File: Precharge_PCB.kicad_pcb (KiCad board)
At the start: 4 copper layers, 146 parts, among them J1 Conn_01x02, J2 Conn_01x02, J3 Conn_01x02, J4 Conn_01x02, J5 Conn_01x08, J6 Conn_01x03, J7 Conn_01x04, J8 Conn_01x04, J9 Conn_01x06, K1 G2RL-1A, K2 G2RL-1A, K3 G9KB-1A, K4 SPU01M-05, Q1 DMN61D8LQ, Q2 DMN61D8LQ, Q3 DMN61D8LQ, Q4 DMN61D8LQ, Q5 DMN61D8LQ, Q6 DMN61D8LQ, Q7 DMN61D8LQ, Q8 DMN61D8LQ, SW1 SW_Push, U1 TPS7B88, U2 MCP1700x-330xxMB, U3 STM32F103C8Tx, U4 SN65HVD1050D, U5 LM393, U6 4N35, U7 AMC1351, U8 AMC1351, U9 TLV6002, Y1 8M

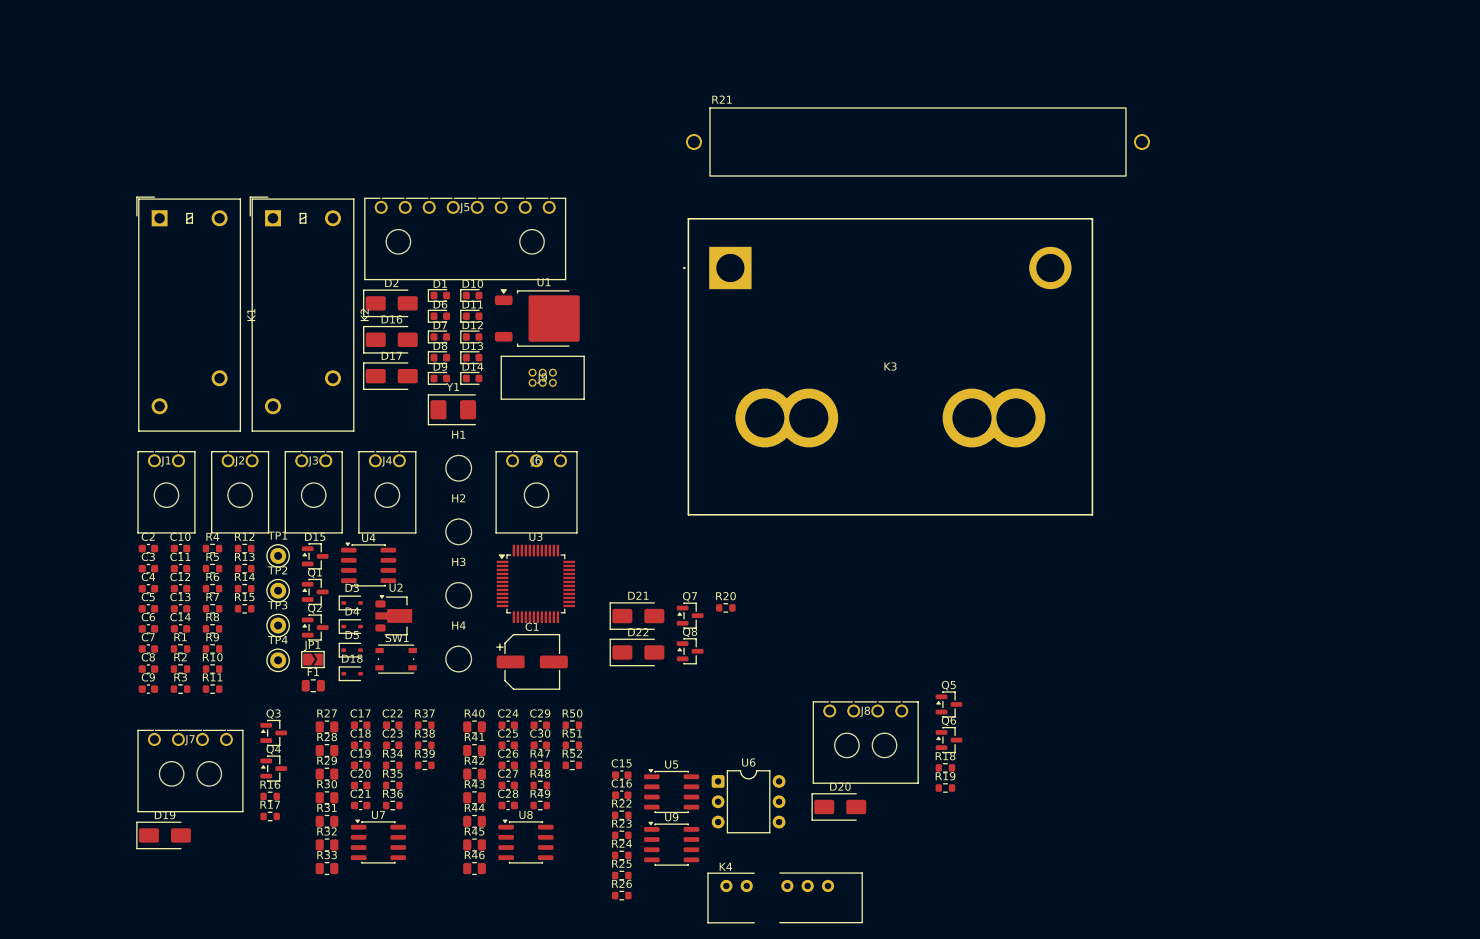
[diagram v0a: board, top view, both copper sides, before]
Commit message: Revision A
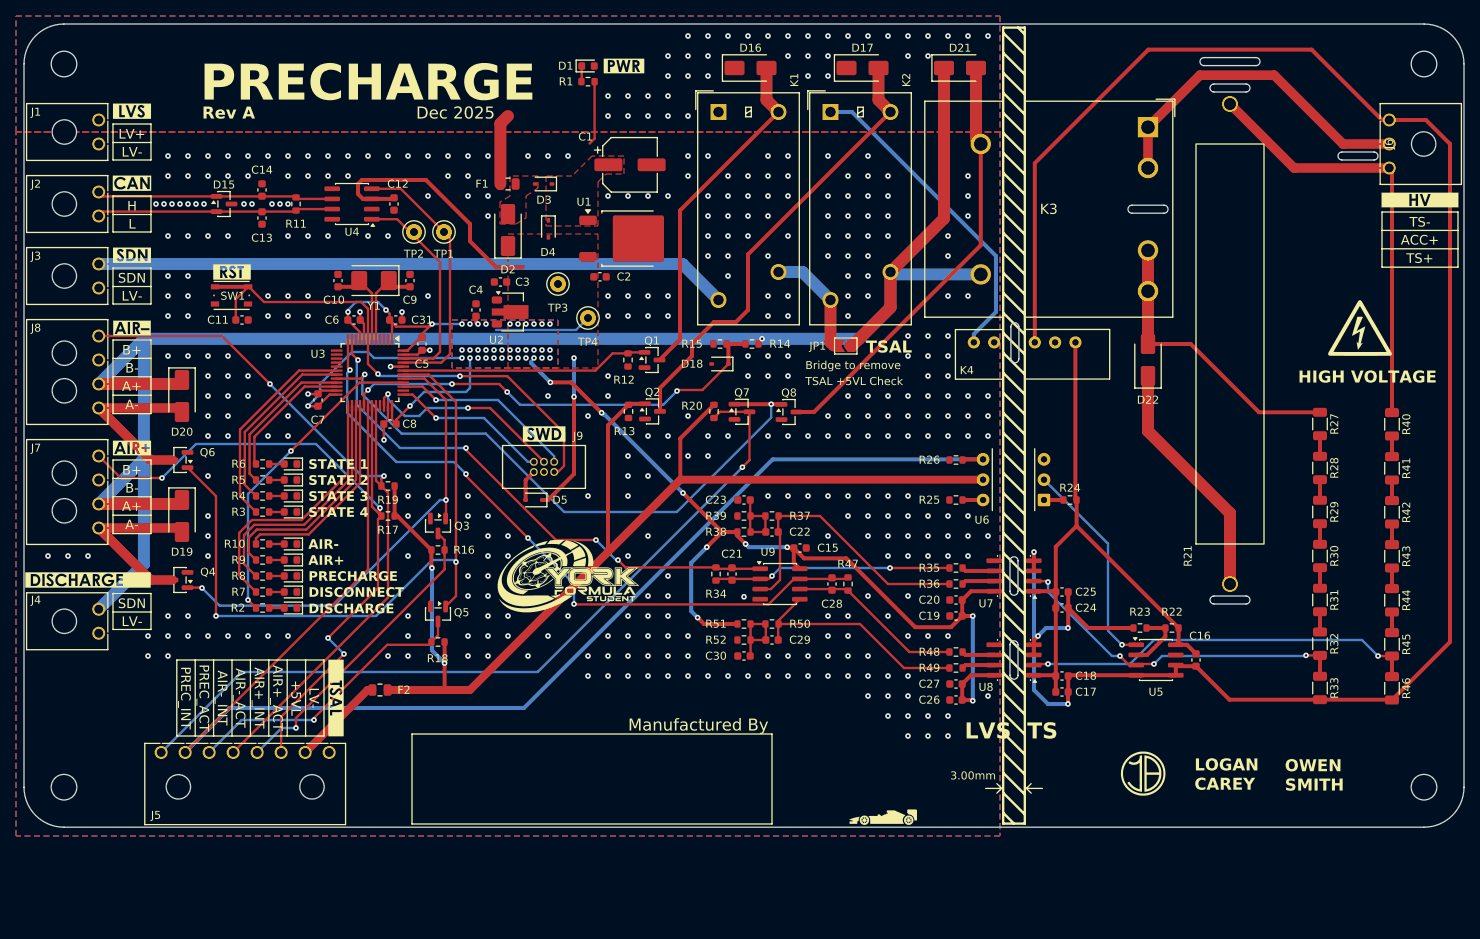
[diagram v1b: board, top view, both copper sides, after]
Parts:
- added C31: 1u, Capacitor_SMD:C_0603_1608Metric, F.Cu at (103.5, 68.0)
- added F2: Polyfuse, Capacitor_SMD:C_0805_2012Metric, F.Cu at (101.5, 114.2)
- added G***: LOGO, LOGO, F.Cu at (224.0, 69.0)
- added G***: LOGO, LOGO, F.Cu at (125.0, 100.0)
- added G***: LOGO, MyLibrary:Logo, F.Cu at (196.9, 124.7)
- added G***: LOGO, MyLibrary:Logo, B.Cu at (139.4, 125.8)
- added G***: LOGO, LOGO, B.Cu at (208.4, 124.0)
- added G***: LOGO, LOGO, B.Cu at (224.0, 69.0)
- added kibuzzard-6910BB45: G***, kibuzzard-6910BB45, F.Cu at (83.0, 62.0)
- added kibuzzard-6910BB76: G***, kibuzzard-6910BB76, F.Cu at (122.0, 82.2)
- added kibuzzard-694056F2: G***, kibuzzard-694056F2, F.Cu at (70.5, 41.9)
- added kibuzzard-694056F9: G***, kibuzzard-694056F9, F.Cu at (70.5, 50.9)
- added kibuzzard-69405726: G***, kibuzzard-69405726, F.Cu at (132.0, 36.2)
- added kibuzzard-69405880: G***, kibuzzard-69405880, F.Cu at (70.5, 59.9)
- added kibuzzard-694058AC: G***, kibuzzard-694058AC, F.Cu at (70.5, 84.0)
- added kibuzzard-694058D8: G***, kibuzzard-694058D8, F.Cu at (70.5, 69.0)
- added kibuzzard-69405918: G***, kibuzzard-69405918, F.Cu at (65.0, 100.5)
- added kibuzzard-69408760: G***, kibuzzard-69408760, F.Cu at (231.5, 53.0)
- added kibuzzard-6940937D: G***, kibuzzard-6940937D, F.Cu at (96.0, 115.2)
- K3: value G9KB-1A -> G9EJH-1-E; footprint yfs:G9KB-1A -> yfs:G9EJH-1-E
- R27, R28, R29, R30, R31, R32, R33, R40, R41, R42, R43, R44, R45, R46: footprint Resistor_SMD:R_0805_2012Metric -> Resistor_SMD:R_1206_3216Metric
- moved H3 137.7 mm to (232.0, 36.0)
- moved R27 129.8 mm to (219.0, 81.0), turned to -90 degrees
- moved R28 129.1 mm to (219.0, 86.5), turned to -90 degrees
- moved R29 128.4 mm to (219.0, 92.0), turned to -90 degrees
- moved R30 127.8 mm to (219.0, 97.5), turned to -90 degrees
- moved R31 127.2 mm to (219.0, 103.0), turned to -90 degrees
- moved R32 126.6 mm to (219.0, 108.5), turned to -90 degrees
- moved R33 126.2 mm to (219.0, 114.0), turned to -90 degrees
- moved H4 121.7 mm to (232.0, 126.4)
- moved R40 120.8 mm to (228.0, 81.0), turned to -90 degrees
- moved R41 120.0 mm to (228.0, 86.5), turned to -90 degrees
- moved R42 119.3 mm to (228.0, 92.0), turned to -90 degrees
- moved R43 118.6 mm to (228.0, 97.5), turned to -90 degrees
- moved R44 118.0 mm to (228.0, 103.0), turned to -90 degrees
- moved R45 117.4 mm to (228.0, 108.5), turned to -90 degrees
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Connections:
- D6 pad 1: Net-(D6-K) -> GND
- D6 pad 2: /STATUS LED -> Net-(D6-A)
- J5 pad 2: +5VL -> Net-(J5-Pin_2)
- R2 pad 1: GND -> Net-(D6-A)
- R2 pad 2: Net-(D6-K) -> /STATUS LED
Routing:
- net GND1: track 0.00 -> 249.7 mm, vias 0 -> 4
- net SHUTDOWN_FINAL: track 0.00 -> 224.6 mm, vias 0 -> 1
- net +3V3: track 0.00 -> 202.4 mm, vias 0 -> 48
- net PRECHARGE_ACT: track 0.00 -> 170.3 mm
- net +5VL: track 0.00 -> 149.3 mm, vias 0 -> 2
- net PRECHARGE_INT: track 0.00 -> 99.5 mm, vias 0 -> 1
- net AIR-_ACT: track 0.00 -> 96.3 mm, vias 0 -> 2
- net AIR+_ACT: track 0.00 -> 93.1 mm, vias 0 -> 4
- net AIR-_CMD: track 0.00 -> 87.1 mm, vias 0 -> 2
- net /HV Sampling/Tractive System: track 0.00 -> 85.0 mm, vias 0 -> 4
- net SHUTDOWN_IN: track 0.00 -> 79.3 mm
- net PRECHARGE_CMD: track 0.00 -> 76.0 mm, vias 0 -> 2
- net +5VA: track 0.00 -> 74.2 mm
- net /HV Sampling/Accumulator: track 0.00 -> 67.6 mm, vias 0 -> 4
- net /NRST: track 0.00 -> 65.8 mm, vias 0 -> 2
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- added copper zone on B.Cu, net +12V
- added copper zone on F.Cu, net +12V
- added copper zone on B.Cu, net +3V3
- added copper zone on F.Cu, net +3V3
- added copper zone on F.Cu, net +5V
- added copper zone on B.Cu, net GND
- added copper zone on F.Cu, net GND
- added copper zone on F.Cu, net Net-(D2-A2)
- added copper zone on F.Cu, net Net-(D3-K)
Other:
- board outline added: 180 x 100.4 mm
- copper layers 4 -> 2
- board text added: "+5VL"
- board text added: "3.00mm"
- board text added: "A+"
- board text added: "A-"
- board text added: "ACC+"
- board text added: "AIR+"
- board text added: "AIR+_ACT"
- board text added: "AIR+_INT"
- board text added: "AIR-"
- board text added: "AIR-_ACT"
- board text added: "AIR-_INT"
- board text added: "B+"
- board text added: "B-"
- board text added: "Bridge to remove"
- board text added: "DISCHARGE"
- board text added: "DISCONNECT"
- board text added: "Dec 2025"
- board text added: "H"
- board text added: "HIGH VOLTAGE"
- board text added: "L"
- board text added: "LOGAN CAREY"
- board text added: "LV+"
- board text added: "LV-"
- board text added: "LVS"
- board text added: "Manufactured By"
- board text added: "OWEN SMITH"
- board text added: "PRECHARGE"
- board text added: "PREC_ACT"
- board text added: "PREC_INT"
- board text added: "Rev A"
- board text added: "SDN"
- board text added: "STATE 1"
- board text added: "STATE 2"
- board text added: "STATE 3"
- board text added: "STATE 4"
- board text added: "TS"
- board text added: "TS+"
- board text added: "TS-"
- board text added: "TSAL"
- board text added: "TSAL +5VL Check"
